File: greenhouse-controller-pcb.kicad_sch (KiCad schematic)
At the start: 12 parts, among them J1 JTAG Interface, SW1 RESET, SW2 Boot mode, U6 CP2102N-Axx-xQFN28

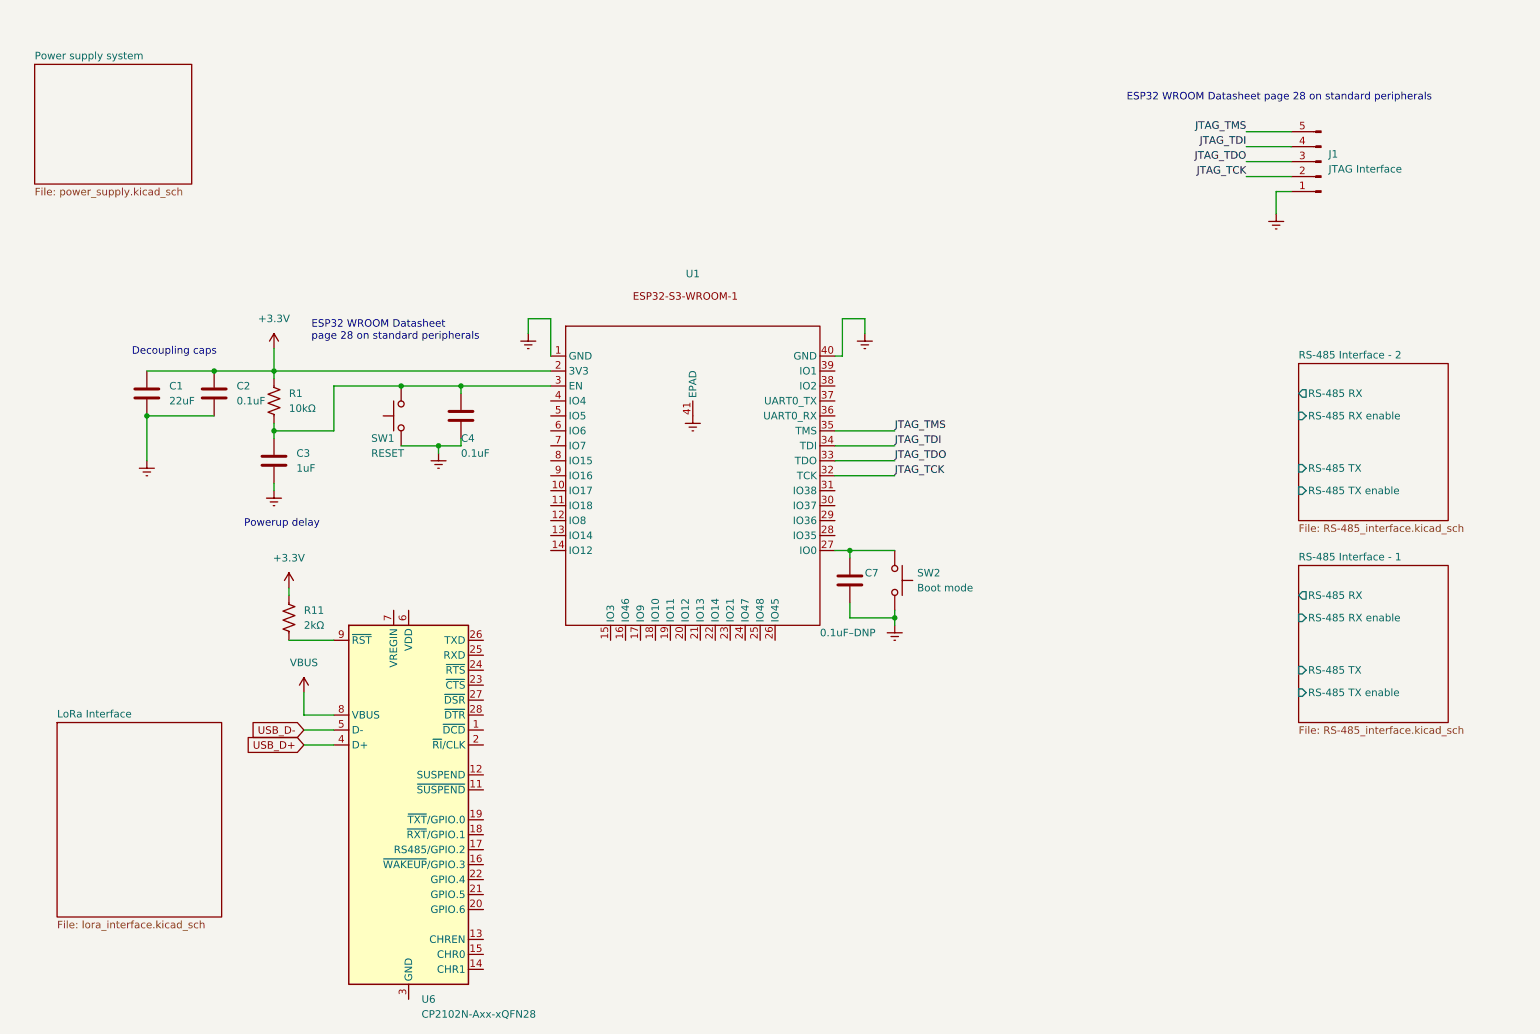
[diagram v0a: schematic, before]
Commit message: version 1
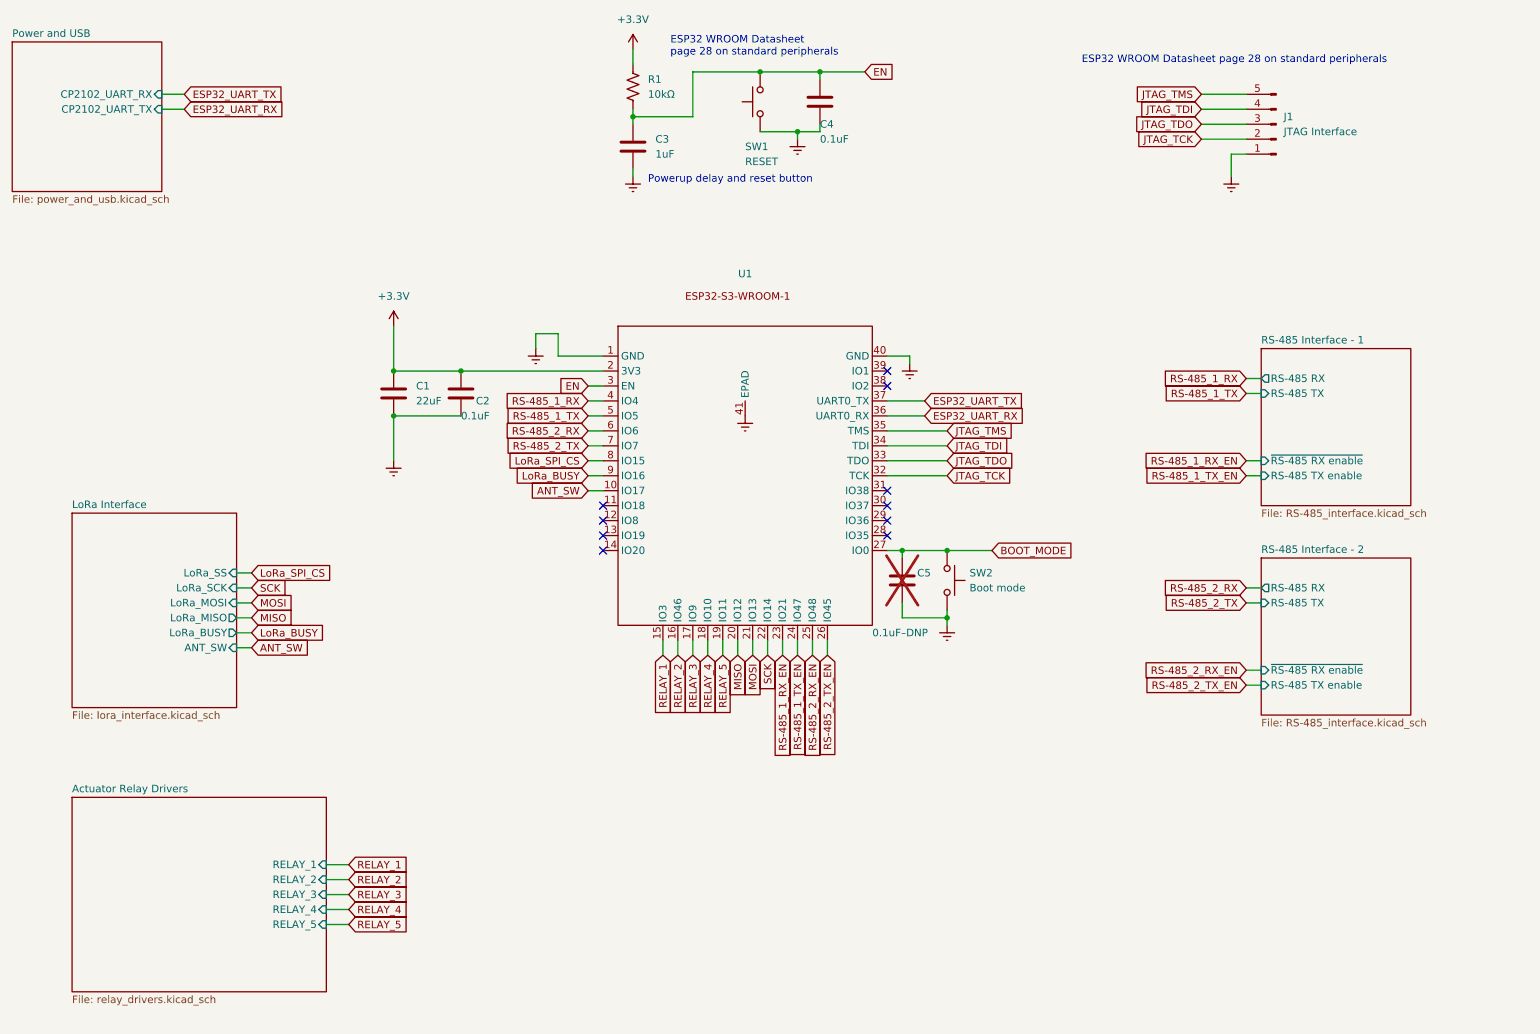
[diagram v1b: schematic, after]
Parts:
- removed R11: 2kΩ, symbol Device:R_US
- removed U6: CP2102N-Axx-xQFN28, Package_DFN_QFN:QFN-28-1EP_5x5mm_P0.5mm_EP3.35x3.35mm, symbol Interface_USB:CP2102N-Axx-xQFN28
- C1, C2, C3, C4: footprint (none) -> Capacitor_SMD:C_0805_2012Metric_Pad1.18x1.45mm_HandSolder
- C5: renamed from C7; now not fitted; now left out of the parts list
- R1: footprint (none) -> Resistor_SMD:R_0805_2012Metric_Pad1.20x1.40mm_HandSolder
- SW1, SW2: footprint (none) -> Library:SW4_PTS815 SJM 250 SMTR LFS_CNK
- U1: footprint (none) -> Library:ESP32-S3-WROOM-1_EXP
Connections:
- net EN: now reaches C3.1, C4.1, R1.2, SW1.2, U1.3 (EN)
- net ANT_SW: now reaches U1.10 (IO17)
- net RELAY_1: now reaches U1.15 (IO3)
- net RELAY_2: now reaches U1.16 (IO46)
- net RELAY_3: now reaches U1.17 (IO9)
- net RELAY_4: now reaches U1.18 (IO10)
- net RELAY_5: now reaches U1.19 (IO11)
- net MISO: now reaches U1.20 (IO12)
- net MOSI: now reaches U1.21 (IO13)
- net SCK: now reaches U1.22 (IO14)
- net RS-485_1_RX_EN: now reaches U1.23 (IO21)
- net RS-485_1_TX_EN: now reaches U1.24 (IO47)
- net RS-485_2_RX_EN: now reaches U1.25 (IO48)
- net RS-485_2_TX_EN: now reaches U1.26 (IO45)
- net BOOT_MODE: now reaches C5.1, SW2.1, U1.27 (IO0)
- net ESP32_UART_RX: now reaches U1.36 (UART0_RX)
- net ESP32_UART_TX: now reaches U1.37 (UART0_TX)
- net RS-485_1_RX: now reaches U1.4 (IO4)
- net RS-485_1_TX: now reaches U1.5 (IO5)
- net RS-485_2_RX: now reaches U1.6 (IO6)
- net RS-485_2_TX: now reaches U1.7 (IO7)
- net LoRa_SPI_CS: now reaches U1.8 (IO15)
- net LoRa_BUSY: now reaches U1.9 (IO16)
- no-connect marks 0 -> 10
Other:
- removed sheet Power supply system
- added sheet Actuator Relay Drivers (relay_drivers.kicad_sch)
- added sheet Power and USB (power_and_usb.kicad_sch)
- sheet LoRa Interface ports: added ANT_SW, LoRa_BUSY, LoRa_MISO, LoRa_MOSI, LoRa_SCK, LoRa_SS; removed none
- sheet RS-485 Interface - 1 ports: added ~{RS-485 RX enable}; removed RS-485 RX enable
- sheet RS-485 Interface - 2 ports: added ~{RS-485 RX enable}; removed RS-485 RX enable
- note added: "Powerup delay and reset button"
- note removed: "Decoupling caps"
- note removed: "Powerup delay"
- company: (none) -> Texas A&M ECEN Capstone
- title: (none) -> Greenhouse Central Controller
- moved on the sheet: C1, C2, J1, SW2, U1
